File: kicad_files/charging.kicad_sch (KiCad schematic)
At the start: 43 parts, among them Q1 AO3400A, Q2 AO3400A, Q3 AO3401A, Q5 Q_PMOS, Q6 AO3401A, U2 BQ24172RGYR, U3 CYPD3177-24LQ

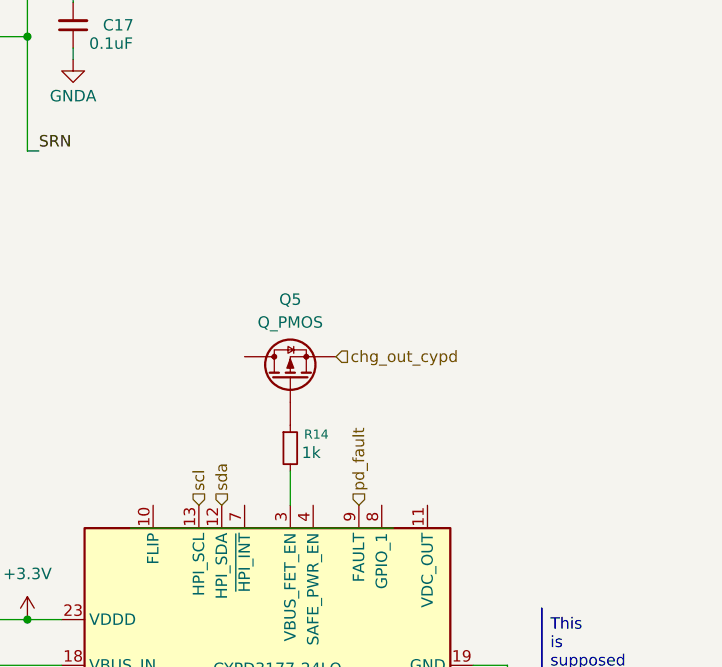
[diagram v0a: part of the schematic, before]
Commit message: copying from reference
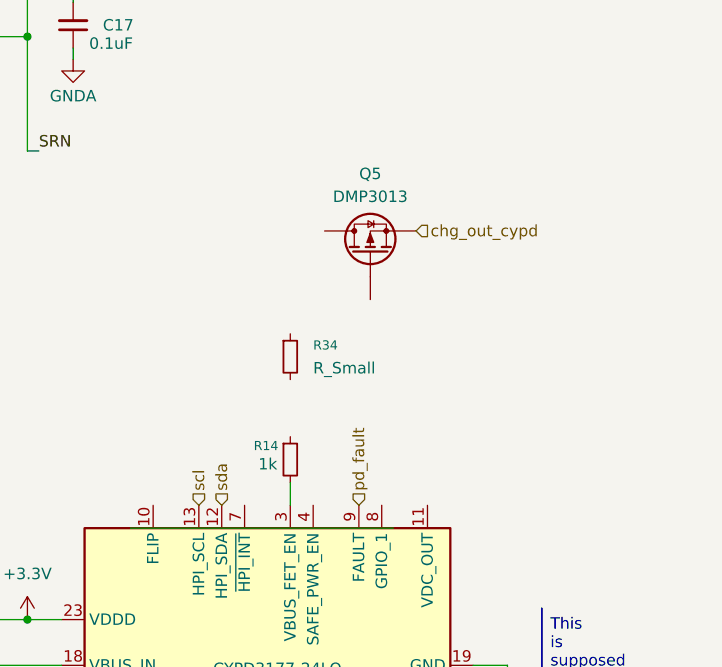
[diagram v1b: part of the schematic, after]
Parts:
- added R34: R_Small, symbol R_Small:R_Small
- Q5: value Q_PMOS -> DMP3013
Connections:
- net at Q5.G: no longer R14.1
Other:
- moved on the sheet: Q5, R14
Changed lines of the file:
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@@
 	(wire
 		(pts
-			(xy 237.49 95.25) (xy 237.49 99.06)
+			(xy 237.49 96.52) (xy 237.49 99.06)
 		)
 		(stroke
@@
 	(hierarchical_label "chg_out_cypd"
 		(shape input)
-		(at 242.57 82.55 0)
+		(at 251.46 68.58 0)
 		(effects
 			(font
@@
 	)
 	(symbol
+		(lib_id "R_Small:R_Small")
+		(at 237.49 82.55 0)
+		(unit 1)
+		(body_style 1)
+		(exclude_from_sim no)
+		(in_bom yes)
+		(on_board yes)
+		(in_pos_files yes)
+		(dnp no)
+		(fields_autoplaced yes)
+		(property "Reference" "R34"
+			(at 240.03 81.2799 0)
+			(show_name no)
+			(do_not_autoplace no)
+			(effects
+				(font
+					(size 1.016 1.016)
+				)
+				(justify left)
+			)
+		)
+		(property "Value" "R_Small"
+			(at 240.03 83.8199 0)
+			(show_name no)
+			(do_not_autoplace no)
+			(effects
+				(font
+					(size 1.27 1.27)
+				)
+				(justify left)
+			)
+		)
+		(property "Footprint" ""
+			(at 237.49 82.55 0)
+			(hide yes)
+			(show_name no)
+			(do_not_autoplace no)
+			(effects
+				(font
+					(size 1.27 1.27)
+				)
+			)
+		)
+		(property "Datasheet" ""
+			(at 237.49 82.55 0)
+			(hide yes)
+			(show_name no)
+			(do_not_autoplace no)
+			(effects
+				(font
+					(size 1.27 1.27)
+				)
+			)
+		)
+		(property "Description" "Resistor, small symbol"
+			(at 237.49 82.55 0)
+			(hide yes)
+			(show_name no)
+			(do_not_autoplace no)
+			(effects
+				(font
+					(size 1.27 1.27)
+				)
+			)
+		)
+		(pin "2"
+		)
+		(pin "1"
+		)
+		(instances
+			(project "sodiumBMS"
+				(path "/fcdd2084-f4ec-4b1b-b9ac-497c327c0303/6e36d9cc-6a8c-4543-ae7a-077a6a363a91"
+					(reference "R34")
+					(unit 1)
+				)
+			)
+		)
+	)
+	(symbol
 		(lib_id "Device:C_Small")
 		(at 78.74 54.61 0)
@@
 	(symbol
 		(lib_id "Q_PMOS:Q_PMOS")
-		(at 237.49 85.09 90)
+		(at 246.38 71.12 90)
 		(unit 1)
 		(body_style 1)
@@
 		(fields_autoplaced yes)
 		(property "Reference" "Q5"
-			(at 237.49 76.2 90)
+			(at 246.38 62.23 90)
 			(show_name no)
 			(do_not_autoplace no)
@@
 			)
 		)
-		(property "Value" "Q_PMOS"
-			(at 237.49 78.74 90)
+		(property "Value" "DMP3013"
+			(at 246.38 64.77 90)
 			(show_name no)
 			(do_not_autoplace no)
@@
 		)
 		(property "Footprint" ""
-			(at 234.95 80.01 0)
+			(at 243.84 66.04 0)
 			(hide yes)
 			(show_name no)
@@
 		)
 		(property "Datasheet" ""
-			(at 237.49 85.09 0)
+			(at 246.38 71.12 0)
 			(hide yes)
 			(show_name no)
@@
 		)
 		(property "Description" "P-MOSFET transistor"
-			(at 237.49 85.09 0)
+			(at 246.38 71.12 0)
 			(hide yes)
 			(show_name no)
@@
 	(symbol
 		(lib_id "R_Small:R_Small")
-		(at 237.49 92.71 0)
+		(at 237.49 93.98 0)
 		(unit 1)
 		(body_style 1)
@@
 		(dnp no)
 		(property "Reference" "R14"
-			(at 239.014 91.186 0)
+			(at 233.426 92.456 0)
 			(show_name no)
 			(do_not_autoplace no)
@@
 		)
 		(property "Value" "1k"
-			(at 238.76 93.218 0)
+			(at 233.934 94.488 0)
 			(show_name no)
 			(do_not_autoplace no)
@@
 		)
 		(property "Footprint" ""
-			(at 237.49 92.71 0)
+			(at 237.49 93.98 0)
 			(hide yes)
 			(show_name no)
@@
 		)
 		(property "Datasheet" ""
-			(at 237.49 92.71 0)
+			(at 237.49 93.98 0)
 			(hide yes)
 			(show_name no)
@@
 		)
 		(property "Description" "Resistor, small symbol"
-			(at 237.49 92.71 0)
+			(at 237.49 93.98 0)
 			(hide yes)
 			(show_name no)
